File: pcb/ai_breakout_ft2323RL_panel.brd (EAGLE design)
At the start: 49.9 x 25.5 mm, 42 parts, among them IC1 FT2332RL, IC2 FT2332RL, IC3 FT2332RL, J1 1X06LONG, J2 1X06LONG, J3 1X06LONG

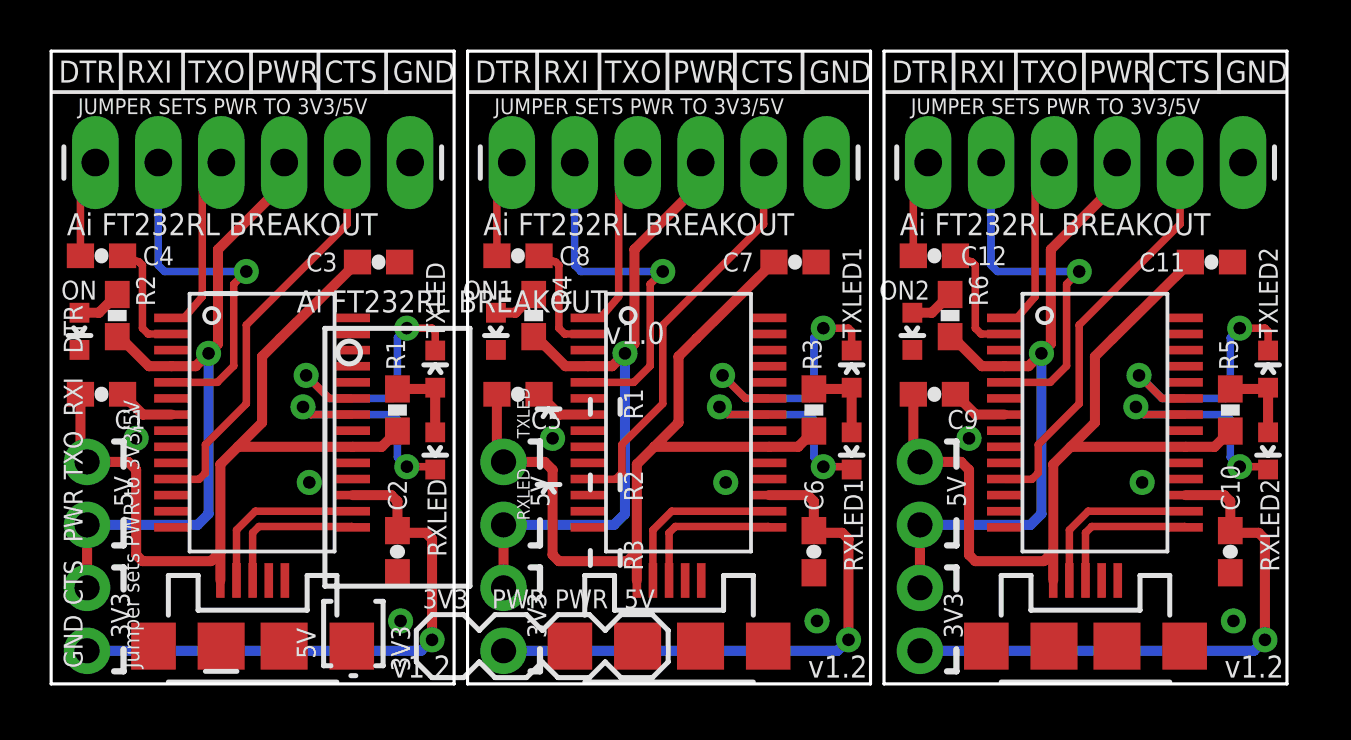
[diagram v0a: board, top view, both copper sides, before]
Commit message: Updated BOM
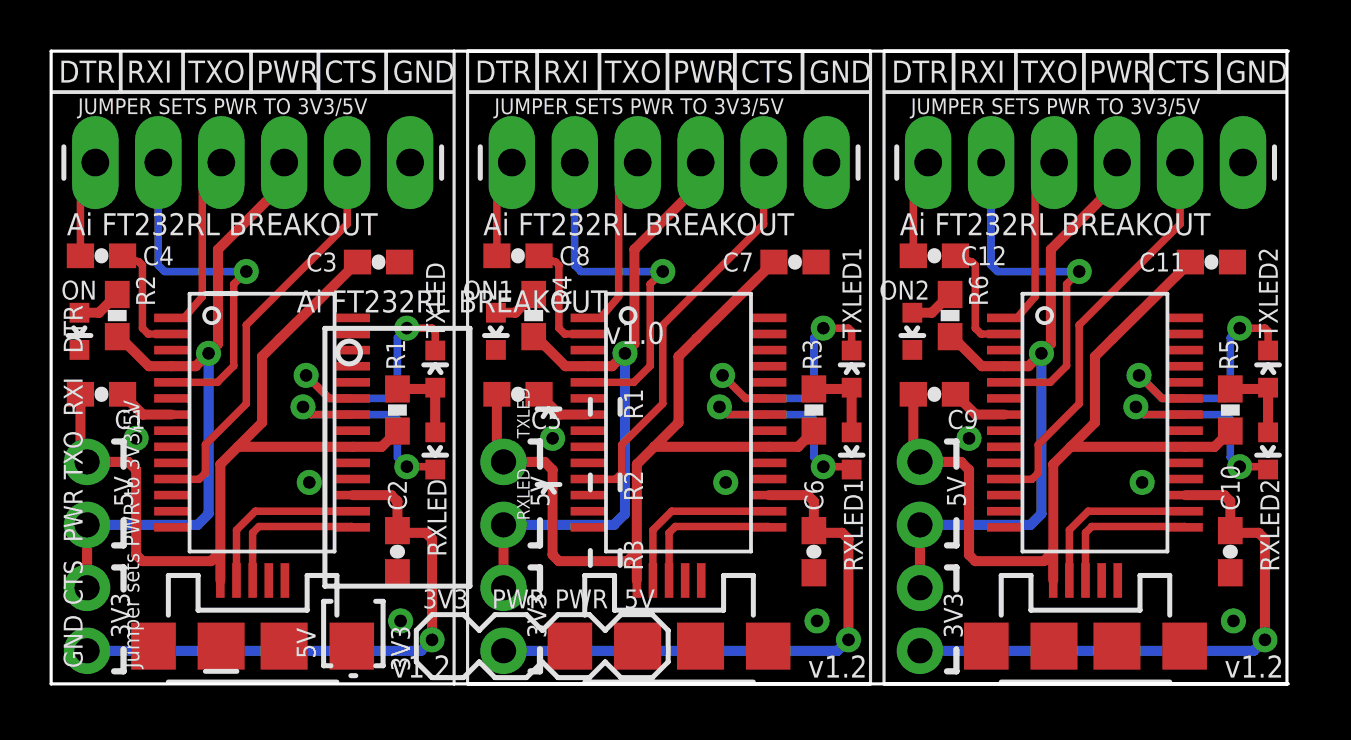
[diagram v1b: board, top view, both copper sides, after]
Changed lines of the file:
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@@
 <setting verticaltext="up"/>
 </settings>
-<grid distance="0.1" unitdist="mm" unit="mm" style="lines" multiple="1" display="yes" altdistance="0.025" altunitdist="inch" altunit="inch"/>
+<grid distance="5" unitdist="mil" unit="mil" style="lines" multiple="1" display="yes" altdistance="0.025" altunitdist="inch" altunit="inch"/>
 <layers>
 <layer number="1" name="Top" color="4" fill="1" visible="yes" active="yes"/>
@@
 <layer number="123" name="tTestmark" color="7" fill="1" visible="yes" active="yes"/>
 <layer number="124" name="bTestmark" color="7" fill="1" visible="yes" active="yes"/>
-<layer number="125" name="_tNames" color="14" fill="1" visible="yes" active="yes"/>
-<layer number="126" name="_bNames" color="7" fill="1" visible="yes" active="yes"/>
+<layer number="125" name="_tNames" color="14" fill="1" visible="no" active="yes"/>
+<layer number="126" name="_bNames" color="7" fill="1" visible="no" active="yes"/>
 <layer number="127" name="_tValues" color="7" fill="1" visible="yes" active="yes"/>
 <layer number="128" name="_bValues" color="7" fill="1" visible="yes" active="yes"/>
@@
 <board>
 <plain>
-<wire x1="0" y1="25.527" x2="0" y2="0" width="0.127" layer="20"/>
 <wire x1="0" y1="0" x2="16.256" y2="0" width="0.127" layer="20"/>
-<wire x1="16.256" y1="0" x2="16.256" y2="25.527" width="0.127" layer="20"/>
+<wire x1="16.256" y1="0" x2="16.256" y2="25.527" width="0.127" layer="21"/>
 <wire x1="16.256" y1="25.527" x2="0" y2="25.527" width="0.127" layer="20"/>
 <text x="5.5372" y="24.257" size="0.889" layer="21" font="vector" ratio="15">TXO</text>
@@
 <text x="15.18399375" y="8.271409375" size="0.762" layer="125" ratio="15" rot="R270">RXLED</text>
 <text x="15.886403125" y="13.953590625" size="0.762" layer="125" ratio="15" rot="R90">TXLED</text>
-<wire x1="16.8" y1="25.527" x2="16.8" y2="0" width="0.127" layer="20"/>
+<wire x1="16.8" y1="25.527" x2="16.8" y2="0" width="0.127" layer="21"/>
 <wire x1="16.8" y1="0" x2="33.056" y2="0" width="0.127" layer="20"/>
-<wire x1="33.056" y1="0" x2="33.056" y2="25.527" width="0.127" layer="20"/>
+<wire x1="33.056" y1="0" x2="33.056" y2="25.527" width="0.127" layer="21"/>
 <wire x1="33.056" y1="25.527" x2="16.8" y2="25.527" width="0.127" layer="20"/>
 <text x="22.3372" y="24.257" size="0.889" layer="21" font="vector" ratio="15">TXO</text>
@@
 <text x="31.98399375" y="8.271409375" size="0.762" layer="125" ratio="15" rot="R270">RXLED</text>
 <text x="32.686403125" y="13.953590625" size="0.762" layer="125" ratio="15" rot="R90">TXLED</text>
-<wire x1="33.6" y1="25.527" x2="33.6" y2="0" width="0.127" layer="20"/>
+<wire x1="33.6" y1="25.527" x2="33.6" y2="0" width="0.127" layer="21"/>
 <wire x1="33.6" y1="0" x2="49.856" y2="0" width="0.127" layer="20"/>
 <wire x1="49.856" y1="0" x2="49.856" y2="25.527" width="0.127" layer="20"/>
@@
 <wire x1="16.528" y1="0" x2="16.528" y2="25.5" width="0.2" layer="125"/>
 <wire x1="33.328" y1="0" x2="33.328" y2="25.5" width="0.2" layer="125"/>
+<wire x1="16.256" y1="0" x2="49.911" y2="0" width="0.127" layer="20"/>
+<wire x1="49.911" y1="25.527" x2="16.256" y2="25.527" width="0.127" layer="20"/>
+<wire x1="0" y1="25.527" x2="0" y2="0" width="0.127" layer="20"/>
 </plain>
 <attributes>
